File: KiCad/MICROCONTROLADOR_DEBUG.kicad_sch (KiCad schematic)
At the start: 9 parts, among them U7 PIC24HJ128GP504-I_PT, Y1 8MHz

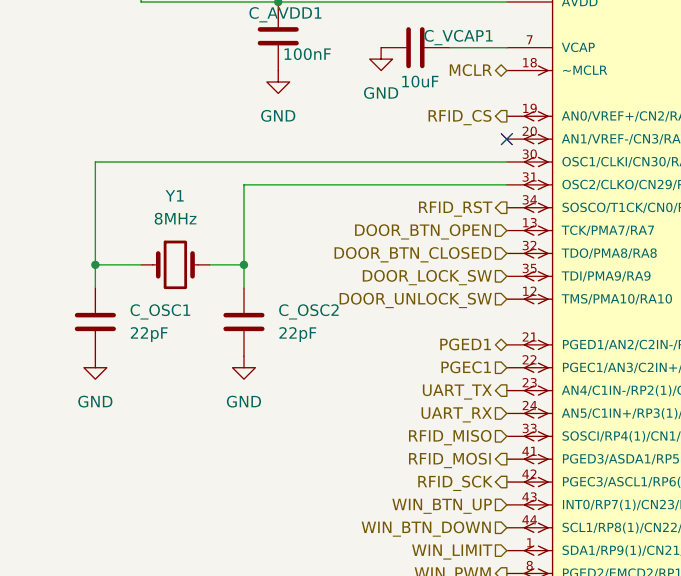
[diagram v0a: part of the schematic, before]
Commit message: Inputs
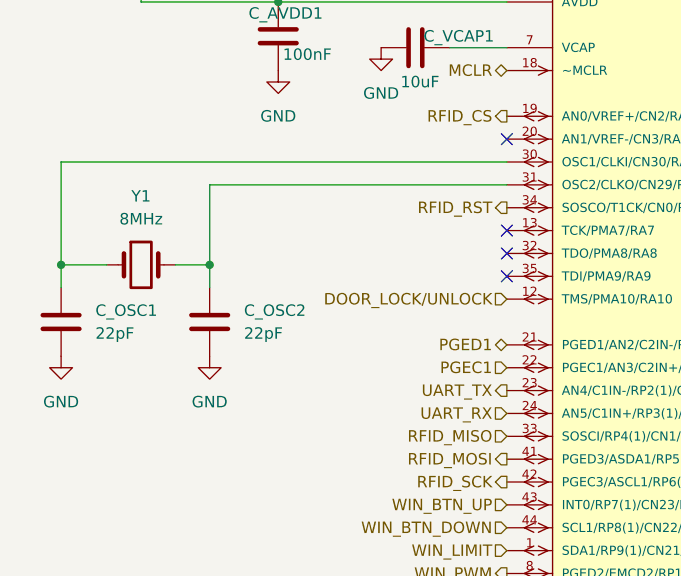
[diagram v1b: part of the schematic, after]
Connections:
- net DOOR_BTN_CLOSED: no longer names the net of U7.32 (TDO/PMA8/RA8)
- net DOOR_BTN_OPEN: no longer names the net of U7.13 (TCK/PMA7/RA7)
- net DOOR_LOCK_SW: no longer names the net of U7.35 (TDI/PMA9/RA9)
- net DOOR_UNLOCK_SW renamed DOOR_LOCK/UNLOCK
- no-connect marks 2 -> 5
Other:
- moved on the sheet: C_OSC1, C_OSC2, Y1
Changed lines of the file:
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@@
 	)
 	(junction
-		(at 64.77 74.93)
+		(at 60.96 74.93)
 		(diameter 0)
 		(color 0 0 0 0)
@@
 	)
 	(junction
-		(at 48.26 74.93)
+		(at 44.45 74.93)
 		(diameter 0)
 		(color 0 0 0 0)
@@
 	)
 	(no_connect
+		(at 93.98 71.12)
+	)
+	(no_connect
 		(at 93.98 60.96)
+	)
+	(no_connect
+		(at 93.98 73.66)
+	)
+	(no_connect
+		(at 93.98 76.2)
 	)
 	(no_connect
@@
 	(wire
 		(pts
-			(xy 48.26 74.93) (xy 53.34 74.93)
+			(xy 44.45 74.93) (xy 49.53 74.93)
 		)
 		(stroke
@@
 	(wire
 		(pts
-			(xy 64.77 74.93) (xy 64.77 77.47)
+			(xy 60.96 74.93) (xy 60.96 77.47)
 		)
 		(stroke
@@
 	(wire
 		(pts
-			(xy 60.96 74.93) (xy 64.77 74.93)
+			(xy 57.15 74.93) (xy 60.96 74.93)
 		)
 		(stroke
@@
 	(wire
 		(pts
-			(xy 48.26 74.93) (xy 48.26 77.47)
+			(xy 44.45 74.93) (xy 44.45 77.47)
 		)
 		(stroke
@@
 	(wire
 		(pts
-			(xy 48.26 63.5) (xy 48.26 74.93)
+			(xy 44.45 63.5) (xy 44.45 74.93)
 		)
 		(stroke
@@
 	(wire
 		(pts
-			(xy 64.77 66.04) (xy 64.77 74.93)
+			(xy 60.96 66.04) (xy 60.96 74.93)
 		)
 		(stroke
@@
 	(wire
 		(pts
-			(xy 93.98 66.04) (xy 64.77 66.04)
-		)
-		(stroke
-			(width 0)
-			(type default)
-		)
-	)
-	(wire
-		(pts
-			(xy 93.98 63.5) (xy 48.26 63.5)
+			(xy 60.96 66.04) (xy 93.98 66.04)
+		)
+		(stroke
+			(width 0)
+			(type default)
+		)
+	)
+	(wire
+		(pts
+			(xy 44.45 63.5) (xy 93.98 63.5)
 		)
 		(stroke
@@
 		)
 	)
-	(hierarchical_label "DOOR_BTN_OPEN"
-		(shape input)
-		(at 93.98 71.12 180)
-		(effects
-			(font
-				(size 1.27 1.27)
-			)
-			(justify right)
-		)
-	)
 	(hierarchical_label "RFID_CS"
 		(shape output)
@@
 		)
 	)
-	(hierarchical_label "DOOR_BTN_CLOSED"
-		(shape input)
-		(at 93.98 73.66 180)
-		(effects
-			(font
-				(size 1.27 1.27)
-			)
-			(justify right)
-		)
-	)
 	(hierarchical_label "DOOR_LIMIT_CLOSE"
 		(shape input)
@@
 		)
 	)
-	(hierarchical_label "DOOR_LOCK_SW"
-		(shape input)
-		(at 93.98 76.2 180)
-		(effects
-			(font
-				(size 1.27 1.27)
-			)
-			(justify right)
-		)
-	)
 	(hierarchical_label "WIN_PWM"
 		(shape output)
@@
 		)
 	)
-	(hierarchical_label "DOOR_UNLOCK_SW"
+	(hierarchical_label "DOOR_LOCK{slash}UNLOCK"
 		(shape input)
 		(at 93.98 78.74 180)
@@
 	(symbol
 		(lib_id "Device:C")
-		(at 64.77 81.28 0)
+		(at 60.96 81.28 0)
 		(unit 1)
 		(exclude_from_sim no)
@@
 		(fields_autoplaced yes)
 		(property "Reference" "C_OSC2"
-			(at 68.58 80.0099 0)
+			(at 64.77 80.0099 0)
 			(effects
 				(font
@@
 		)
 		(property "Value" "22pF"
-			(at 68.58 82.5499 0)
+			(at 64.77 82.5499 0)
 			(effects
 				(font
@@
 		)
 		(property "Footprint" "Capacitor_SMD:C_0603_1608Metric"
-			(at 65.7352 85.09 0)
+			(at 61.9252 85.09 0)
 			(effects
 				(font
@@
 		)
 		(property "Datasheet" "~"
-			(at 64.77 81.28 0)
+			(at 60.96 81.28 0)
 			(effects
 				(font
@@
 		)
 		(property "Description" "Unpolarized capacitor"
-			(at 64.77 81.28 0)
+			(at 60.96 81.28 0)
 			(effects
 				(font
@@
 	(symbol
 		(lib_id "Device:Crystal")
-		(at 57.15 74.93 0)
+		(at 53.34 74.93 0)
 		(unit 1)
 		(exclude_from_sim no)
@@
 		(fields_autoplaced yes)
 		(property "Reference" "Y1"
-			(at 57.15 67.31 0)
+			(at 53.34 67.31 0)
 			(effects
 				(font
@@
 		)
 		(property "Value" "8MHz"
-			(at 57.15 69.85 0)
+			(at 53.34 69.85 0)
 			(effects
 				(font
@@
 		)
 		(property "Footprint" "Crystal:Crystal_SMD_3225-4Pin_3.2x2.5mm"
-			(at 57.15 74.93 0)
+			(at 53.34 74.93 0)
 			(effects
 				(font
@@
 		)
 		(property "Datasheet" "~"
-			(at 57.15 74.93 0)
+			(at 53.34 74.93 0)
 			(effects
 				(font
@@
 		)
 		(property "Description" "Two pin crystal"
-			(at 57.15 74.93 0)
+			(at 53.34 74.93 0)
 			(effects
 				(font
@@
 	(symbol
 		(lib_id "power:GND")
-		(at 48.26 85.09 0)
+		(at 44.45 85.09 0)
 		(unit 1)
 		(exclude_from_sim no)
@@
 		(fields_autoplaced yes)
 		(property "Reference" "#PWR09"
-			(at 48.26 91.44 0)
+			(at 44.45 91.44 0)
 			(effects
 				(font
@@
 		)
 		(property "Value" "GND"
-			(at 48.26 90.17 0)
+			(at 44.45 90.17 0)
 			(effects
 				(font
@@
 		)
 		(property "Footprint" ""
-			(at 48.26 85.09 0)
+			(at 44.45 85.09 0)
 			(effects
 				(font
@@
 		)
 		(property "Datasheet" ""
-			(at 48.26 85.09 0)
+			(at 44.45 85.09 0)
 			(effects
 				(font
@@
 		)
 		(property "Description" "Power symbol creates a global label with name \"GND\" , ground"
-			(at 48.26 85.09 0)
+			(at 44.45 85.09 0)
 			(effects
 				(font
@@
 	(symbol
 		(lib_id "power:GND")
-		(at 64.77 85.09 0)
+		(at 60.96 85.09 0)
 		(unit 1)
 		(exclude_from_sim no)
@@
 		(fields_autoplaced yes)
 		(property "Reference" "#PWR010"
-			(at 64.77 91.44 0)
+			(at 60.96 91.44 0)
 			(effects
 				(font
@@
 		)
 		(property "Value" "GND"
-			(at 64.77 90.17 0)
+			(at 60.96 90.17 0)
 			(effects
 				(font
@@
 		)
 		(property "Footprint" ""
-			(at 64.77 85.09 0)
+			(at 60.96 85.09 0)
 			(effects
 				(font
@@
 		)
 		(property "Datasheet" ""
-			(at 64.77 85.09 0)
+			(at 60.96 85.09 0)
 			(effects
 				(font
@@
 		)
 		(property "Description" "Power symbol creates a global label with name \"GND\" , ground"
-			(at 64.77 85.09 0)
+			(at 60.96 85.09 0)
 			(effects
 				(font
@@
 	(symbol
 		(lib_id "Device:C")
-		(at 48.26 81.28 0)
+		(at 44.45 81.28 0)
 		(unit 1)
 		(exclude_from_sim no)
@@
 		(fields_autoplaced yes)
 		(property "Reference" "C_OSC1"
-			(at 52.07 80.0099 0)
+			(at 48.26 80.0099 0)
 			(effects
 				(font
@@
 		)
 		(property "Value" "22pF"
-			(at 52.07 82.5499 0)
+			(at 48.26 82.5499 0)
 			(effects
 				(font
@@
 		)
 		(property "Footprint" "Capacitor_SMD:C_0603_1608Metric"
-			(at 49.2252 85.09 0)
+			(at 45.4152 85.09 0)
 			(effects
 				(font
@@
 		)
 		(property "Datasheet" "~"
-			(at 48.26 81.28 0)
+			(at 44.45 81.28 0)
 			(effects
 				(font
@@
 		)
 		(property "Description" "Unpolarized capacitor"
-			(at 48.26 81.28 0)
-			(effects
-				(font
+			(at 44.45 81.28 0)
+			(effects
+				(font
